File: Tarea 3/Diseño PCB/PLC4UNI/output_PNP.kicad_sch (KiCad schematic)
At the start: 21 parts, among them Q5 IRLML0040, Q7 IRLML0040, Q9 IRLML0040

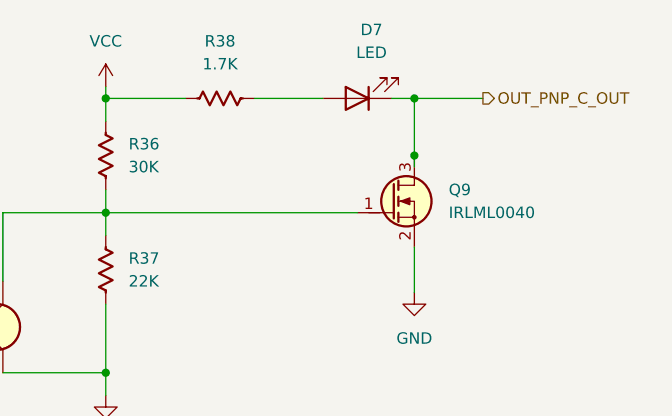
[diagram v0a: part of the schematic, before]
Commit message: Tarea  3
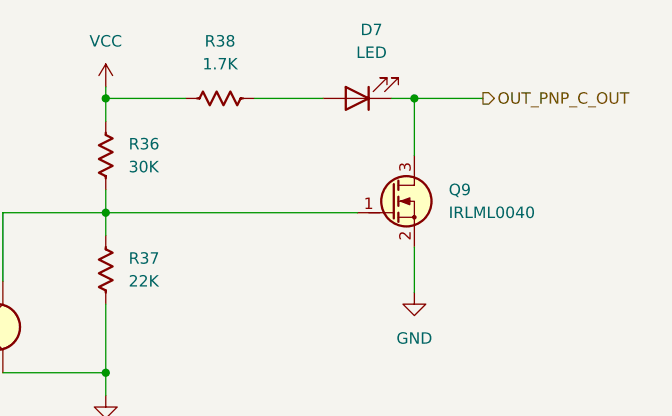
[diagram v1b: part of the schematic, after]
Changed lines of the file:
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@@
+	)
+	(junction
+		(at 233.68 35.56)
+		(diameter 0)
+		(color 0 0 0 0)
 	)
 	(junction
@@
 	)
 	(junction
-		(at 233.68 41.91)
-		(diameter 0)
-		(color 0 0 0 0)
-	)
-	(junction
 		(at 115.57 40.64)
 		(diameter 0)
@@
 		(color 0 0 0 0)
 	)
-	(junction
-		(at 233.68 35.56)
-		(diameter 0)
-		(color 0 0 0 0)
-	)
 	(wire
 		(pts
@@
 	(wire
 		(pts
-			(xy 233.68 41.91) (xy 233.68 35.56)
-		)
-		(stroke
-			(width 0)
-			(type default)
-		)
-	)
-	(wire
-		(pts
 			(xy 115.57 40.64) (xy 115.57 46.99)
 		)
@@
 	(wire
 		(pts
-			(xy 233.68 43.18) (xy 233.68 41.91)
-		)
-		(stroke
-			(width 0)
-			(type default)
-		)
-	)
-	(wire
-		(pts
 			(xy 180.34 66.04) (xy 180.34 69.85)
 		)
@@
 	(wire
 		(pts
+			(xy 82.55 96.52) (xy 82.55 97.79)
+		)
+		(stroke
+			(width 0)
+			(type default)
+		)
+	)
+	(wire
+		(pts
+			(xy 187.96 48.26) (xy 187.96 55.88)
+		)
+		(stroke
+			(width 0)
+			(type default)
+		)
+	)
+	(wire
+		(pts
+			(xy 116.84 97.79) (xy 124.46 97.79)
+		)
+		(stroke
+			(width 0)
+			(type default)
+		)
+	)
+	(wire
+		(pts
+			(xy 116.84 104.14) (xy 116.84 97.79)
+		)
+		(stroke
+			(width 0)
+			(type default)
+		)
+	)
+	(wire
+		(pts
+			(xy 116.84 114.3) (xy 116.84 119.38)
+		)
+		(stroke
+			(width 0)
+			(type default)
+		)
+	)
+	(wire
+		(pts
+			(xy 71.12 71.12) (xy 71.12 72.39)
+		)
+		(stroke
+			(width 0)
+			(type default)
+		)
+	)
+	(wire
+		(pts
+			(xy 57.15 116.84) (xy 63.5 116.84)
+		)
+		(stroke
+			(width 0)
+			(type default)
+		)
+	)
+	(wire
+		(pts
+			(xy 199.39 58.42) (xy 199.39 66.04)
+		)
+		(stroke
+			(width 0)
+			(type default)
+		)
+	)
+	(wire
+		(pts
+			(xy 82.55 53.34) (xy 109.22 53.34)
+		)
+		(stroke
+			(width 0)
+			(type default)
+		)
+	)
+	(wire
+		(pts
+			(xy 116.84 97.79) (xy 114.3 97.79)
+		)
+		(stroke
+			(width 0)
+			(type default)
+		)
+	)
+	(wire
+		(pts
+			(xy 82.55 72.39) (xy 82.55 76.2)
+		)
+		(stroke
+			(width 0)
+			(type default)
+		)
+	)
+	(wire
+		(pts
+			(xy 82.55 53.34) (xy 82.55 55.88)
+		)
+		(stroke
+			(width 0)
+			(type default)
+		)
+	)
+	(wire
+		(pts
+			(xy 199.39 66.04) (xy 199.39 68.58)
+		)
+		(stroke
+			(width 0)
+			(type default)
+		)
+	)
+	(wire
+		(pts
+			(xy 71.12 110.49) (xy 71.12 118.11)
+		)
+		(stroke
+			(width 0)
+			(type default)
+		)
+	)
+	(wire
+		(pts
+			(xy 82.55 53.34) (xy 71.12 53.34)
+		)
+		(stroke
+			(width 0)
+			(type default)
+		)
+	)
+	(wire
+		(pts
+			(xy 199.39 48.26) (xy 187.96 48.26)
+		)
+		(stroke
+			(width 0)
+			(type default)
+		)
+	)
+	(wire
+		(pts
+			(xy 233.68 52.07) (xy 233.68 57.15)
+		)
+		(stroke
+			(width 0)
+			(type default)
+		)
+	)
+	(wire
+		(pts
+			(xy 82.55 97.79) (xy 82.55 100.33)
+		)
+		(stroke
+			(width 0)
+			(type default)
+		)
+	)
+	(wire
+		(pts
 			(xy 233.68 35.56) (xy 241.3 35.56)
 		)
@@
 	(wire
 		(pts
-			(xy 82.55 96.52) (xy 82.55 97.79)
-		)
-		(stroke
-			(width 0)
-			(type default)
-		)
-	)
-	(wire
-		(pts
-			(xy 187.96 48.26) (xy 187.96 55.88)
-		)
-		(stroke
-			(width 0)
-			(type default)
-		)
-	)
-	(wire
-		(pts
-			(xy 116.84 97.79) (xy 124.46 97.79)
-		)
-		(stroke
-			(width 0)
-			(type default)
-		)
-	)
-	(wire
-		(pts
-			(xy 116.84 104.14) (xy 116.84 97.79)
-		)
-		(stroke
-			(width 0)
-			(type default)
-		)
-	)
-	(wire
-		(pts
-			(xy 116.84 114.3) (xy 116.84 119.38)
-		)
-		(stroke
-			(width 0)
-			(type default)
-		)
-	)
-	(wire
-		(pts
-			(xy 71.12 71.12) (xy 71.12 72.39)
-		)
-		(stroke
-			(width 0)
-			(type default)
-		)
-	)
-	(wire
-		(pts
-			(xy 57.15 116.84) (xy 63.5 116.84)
-		)
-		(stroke
-			(width 0)
-			(type default)
-		)
-	)
-	(wire
-		(pts
-			(xy 199.39 58.42) (xy 199.39 66.04)
-		)
-		(stroke
-			(width 0)
-			(type default)
-		)
-	)
-	(wire
-		(pts
-			(xy 82.55 53.34) (xy 109.22 53.34)
-		)
-		(stroke
-			(width 0)
-			(type default)
-		)
-	)
-	(wire
-		(pts
-			(xy 116.84 97.79) (xy 114.3 97.79)
-		)
-		(stroke
-			(width 0)
-			(type default)
-		)
-	)
-	(wire
-		(pts
-			(xy 82.55 72.39) (xy 82.55 76.2)
-		)
-		(stroke
-			(width 0)
-			(type default)
-		)
-	)
-	(wire
-		(pts
-			(xy 82.55 53.34) (xy 82.55 55.88)
-		)
-		(stroke
-			(width 0)
-			(type default)
-		)
-	)
-	(wire
-		(pts
-			(xy 199.39 66.04) (xy 199.39 68.58)
-		)
-		(stroke
-			(width 0)
-			(type default)
-		)
-	)
-	(wire
-		(pts
-			(xy 71.12 110.49) (xy 71.12 118.11)
-		)
-		(stroke
-			(width 0)
-			(type default)
-		)
-	)
-	(wire
-		(pts
-			(xy 82.55 53.34) (xy 71.12 53.34)
-		)
-		(stroke
-			(width 0)
-			(type default)
-		)
-	)
-	(wire
-		(pts
-			(xy 199.39 48.26) (xy 187.96 48.26)
-		)
-		(stroke
-			(width 0)
-			(type default)
-		)
-	)
-	(wire
-		(pts
-			(xy 233.68 52.07) (xy 233.68 57.15)
-		)
-		(stroke
-			(width 0)
-			(type default)
-		)
-	)
-	(wire
-		(pts
-			(xy 82.55 97.79) (xy 82.55 100.33)
-		)
-		(stroke
-			(width 0)
-			(type default)
-		)
-	)
-	(wire
-		(pts
 			(xy 82.55 97.79) (xy 91.44 97.79)
 		)
@@
 	(wire
 		(pts
+			(xy 233.68 35.56) (xy 233.68 41.91)
+		)
+		(stroke
+			(width 0)
+			(type default)
+		)
+	)
+	(wire
+		(pts
 			(xy 82.55 110.49) (xy 82.55 113.03)
 		)
@@
 	(wire
 		(pts
-			(xy 233.68 35.56) (xy 231.14 35.56)
-		)
-		(stroke
+			(xy 231.14 35.56) (xy 233.68 35.56)
+		)
+		(stroke

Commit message: Tarea 3
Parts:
- D5, D6, D7: footprint (none) -> LED_SMD:LED_0603_1608Metric
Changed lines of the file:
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@@
 			)
 		)
-		(property "Footprint" ""
+		(property "Footprint" "LED_SMD:LED_0603_1608Metric"
 			(at 110.49 40.64 0)
 			(effects
@@
 			)
 		)
-		(property "Footprint" ""
+		(property "Footprint" "LED_SMD:LED_0603_1608Metric"
 			(at 110.49 97.79 0)
 			(effects
@@
 			)
 		)
-		(property "Footprint" ""
+		(property "Footprint" "LED_SMD:LED_0603_1608Metric"
 			(at 227.33 35.56 0)
 			(effects
